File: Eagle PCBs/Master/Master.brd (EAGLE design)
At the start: 87.3 x 36.8 mm, 15 parts

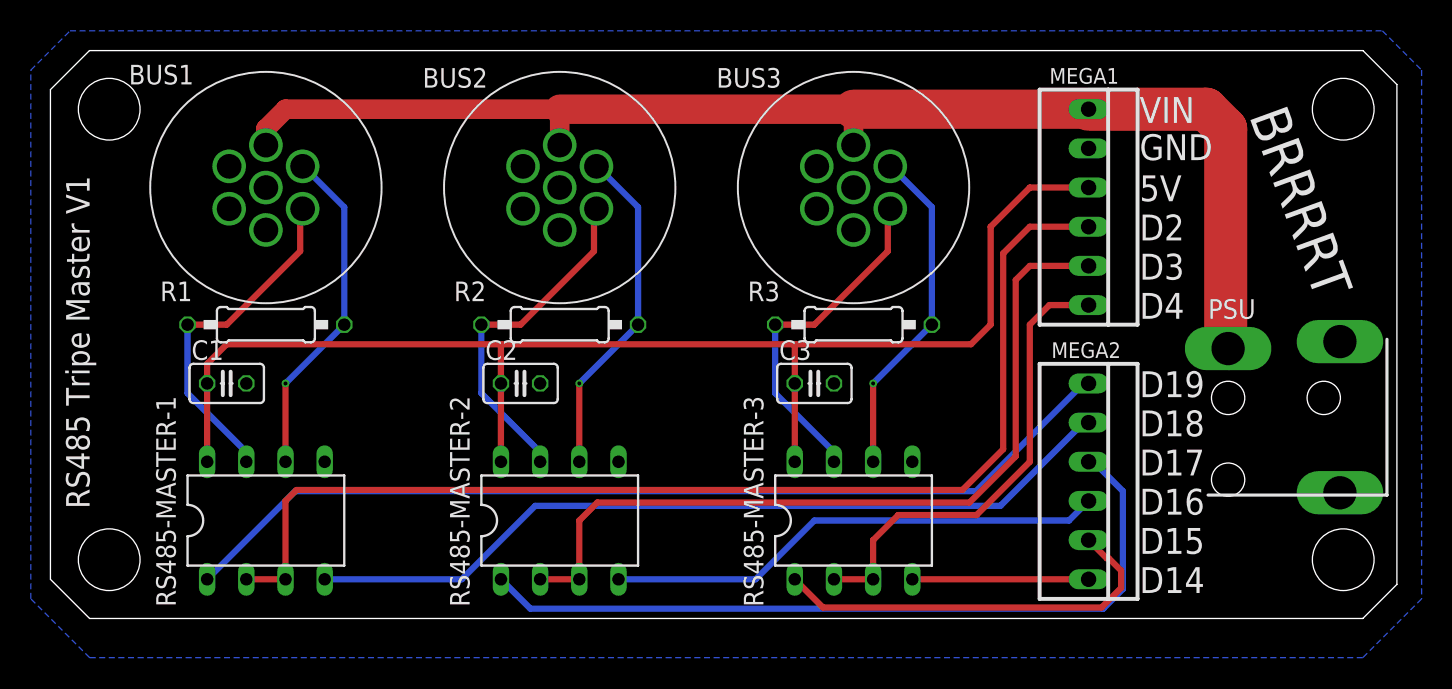
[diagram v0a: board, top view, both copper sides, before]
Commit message: New slave PCB
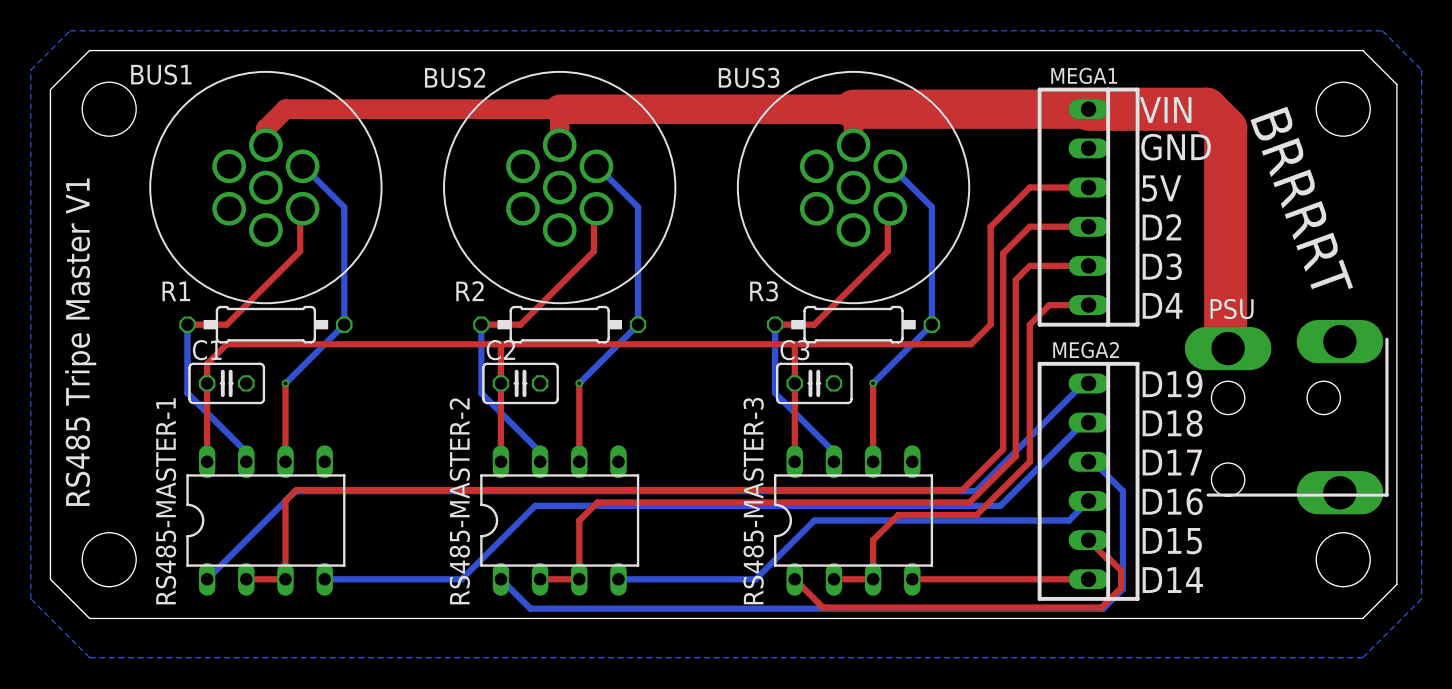
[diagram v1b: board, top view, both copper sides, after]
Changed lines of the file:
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@@
 <setting verticaltext="up"/>
 </settings>
-<grid distance="50" unitdist="mil" unit="mil" style="lines" multiple="1" display="no" altdistance="5" altunitdist="mil" altunit="mil"/>
+<grid distance="50" unitdist="mil" unit="mm" style="lines" multiple="1" display="no" altdistance="5" altunitdist="mil" altunit="mil"/>
 <layers>
 <layer number="1" name="Top" color="4" fill="1" visible="yes" active="yes"/>
@@
 <wire x1="85.1" y1="36.82" x2="2.53" y2="36.82" width="0" layer="20"/>
 <wire x1="2.53" y1="36.82" x2="0" y2="34.29" width="0" layer="20"/>
-<hole x="3.81" y="33.02" drill="4"/>
-<hole x="3.81" y="3.81" drill="4"/>
-<hole x="83.82" y="33.02" drill="4"/>
-<hole x="83.82" y="3.81" drill="4"/>
+<hole x="3.81" y="33.02" drill="3.5"/>
+<hole x="3.81" y="3.81" drill="3.5"/>
+<hole x="83.82" y="33.02" drill="3.5"/>
+<hole x="83.82" y="3.81" drill="3.5"/>
 <text x="70.612" y="32.131" size="1.6764" layer="25">VIN</text>
 <text x="70.612" y="29.718" size="1.6764" layer="25">GND</text>
